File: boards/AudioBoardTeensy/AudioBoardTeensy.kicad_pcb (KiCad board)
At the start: 2 copper layers, 54.5 x 26.4 mm, 12 parts, among them J1 54-00174, J2 Conn_01x10_Pin, J3 Conn_01x10_Pin, J4 DFR0934, U1 Teensy4.0

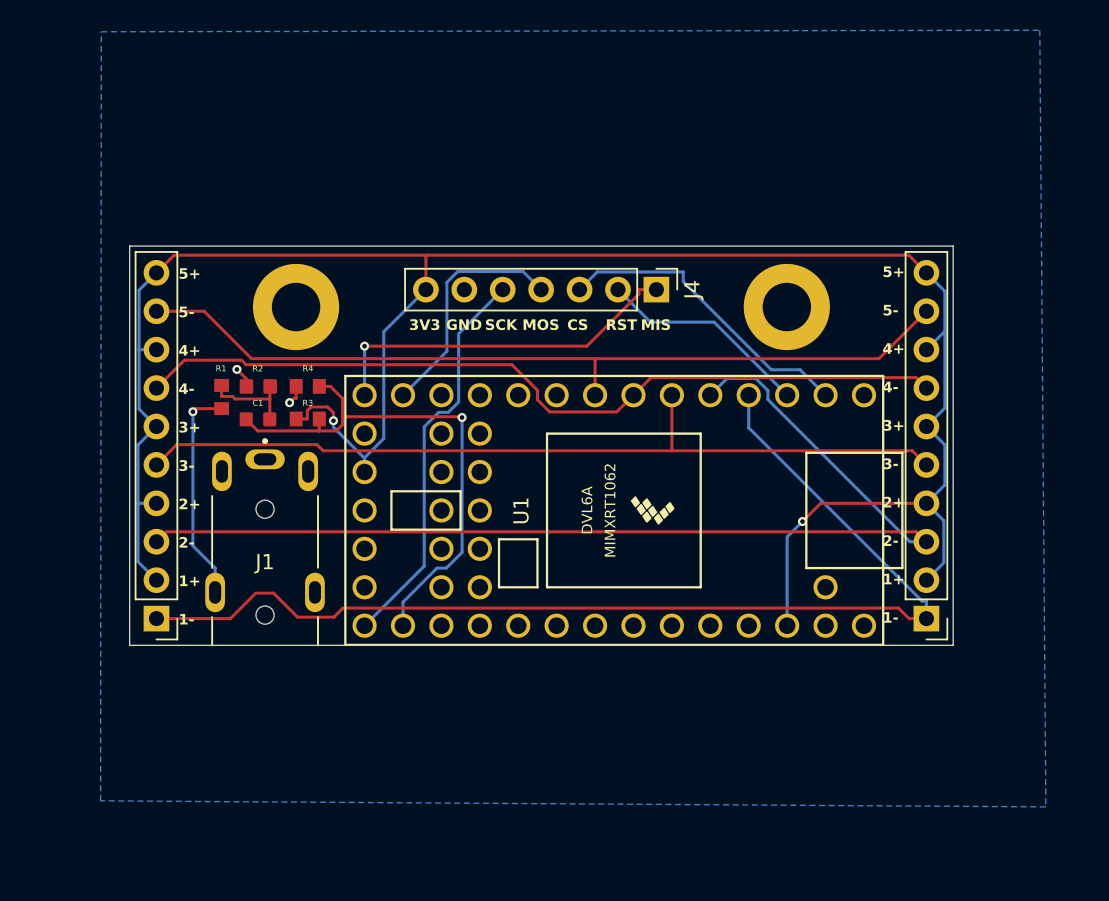
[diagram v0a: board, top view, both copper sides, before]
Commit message: Re-finalize audio board and cleanup
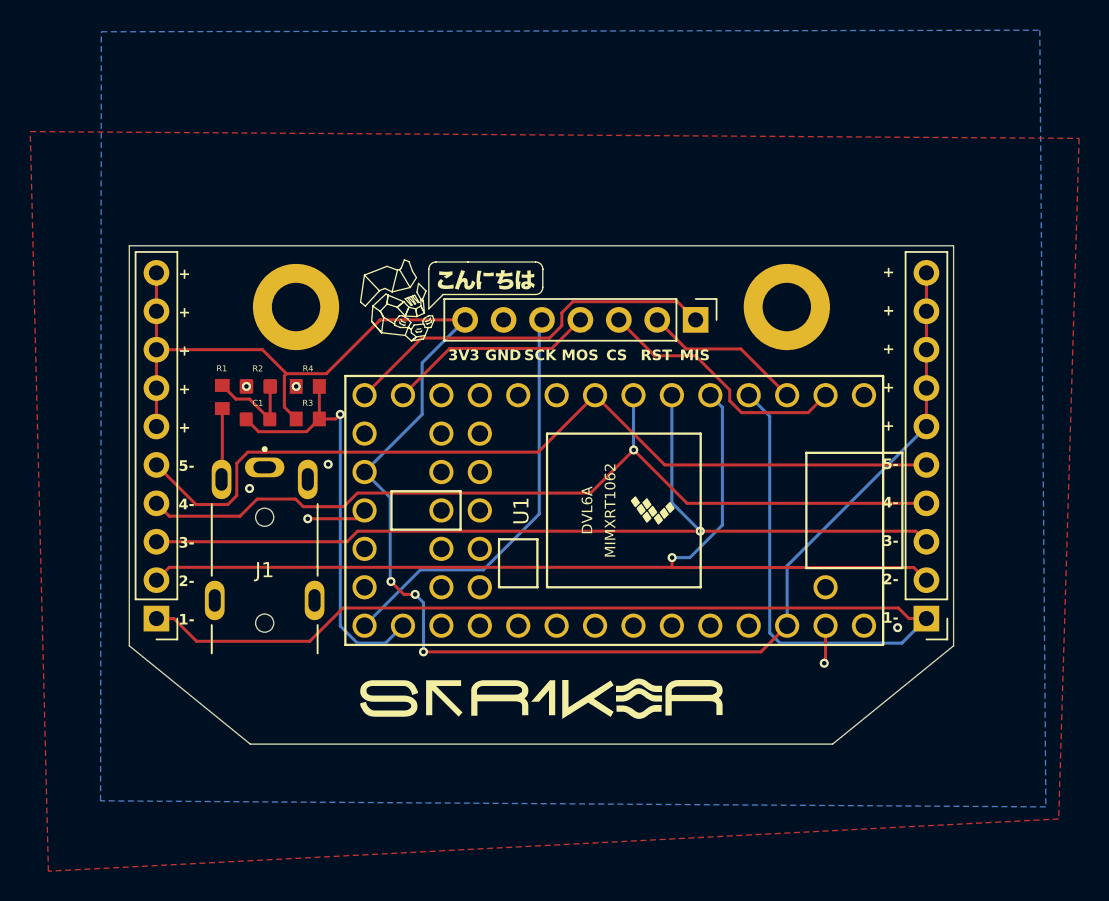
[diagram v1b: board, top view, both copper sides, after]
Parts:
- moved J4 3.28 mm to (150.5, 92.2)
- moved J1 0.53 mm to (122.0, 108.8)
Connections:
- J1 pad 2: GND -> AUDIO
- J1 pad 3: /RING 1 -> GND
- J1 pad 4_1: AUDIO -> /TIP 1
- J2 pad 2: +3V3 -> LED2
- J2 pad 3: LED2 -> LED3
- J2 pad 4: +3V3 -> LED4
- J2 pad 5: LED3 -> LED5
- J2 pad 7: LED4 -> +3V3
- J2 pad 9: LED5 -> +3V3
- J3 pad 2: +3V3 -> LED2
- J3 pad 3: LED2 -> LED3
- J3 pad 4: +3V3 -> LED4
- J3 pad 5: LED3 -> LED5
- J3 pad 7: LED4 -> +3V3
- J3 pad 9: LED5 -> +3V3
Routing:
- net +3V3: track 140.7 -> 114.7 mm, vias 2 -> 3
- net AUDIO: track 14.5 -> 4.71 mm, vias 1 -> 0
- net LED1: track 72.6 -> 80.3 mm
- net A0: track 34.9 -> 28.3 mm
- net LED2: track 71.0 -> 65.4 mm, vias 0 -> 1
- net LED3: track 55.7 -> 61.3 mm, vias 0 -> 1
- net LED4: track 54.7 -> 58.6 mm, vias 0 -> 1
- net GND: track 2.73 -> 6.50 mm, vias 2 -> 7
- net RST: track 14.1 -> 10.7 mm
- net CS: track 20.5 -> 17.1 mm
- net LED5: track 55.9 -> 58.2 mm
- net MOSI: track 15.7 -> 13.8 mm
- net MISO: track 24.3 -> 25.5 mm, vias 1 -> 0
- net SCK: track 26.4 -> 27.5 mm
- added copper zone on F.Cu, net GND
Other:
- board size 54.5 x 26.4 mm -> 54.5 x 33 mm
- board text added: "+"
- board text removed: "1+"
- board text removed: "2+"
- board text removed: "3+"
- board text removed: "4+"
- board text removed: "5+"
